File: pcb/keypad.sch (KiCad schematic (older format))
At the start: 1 part

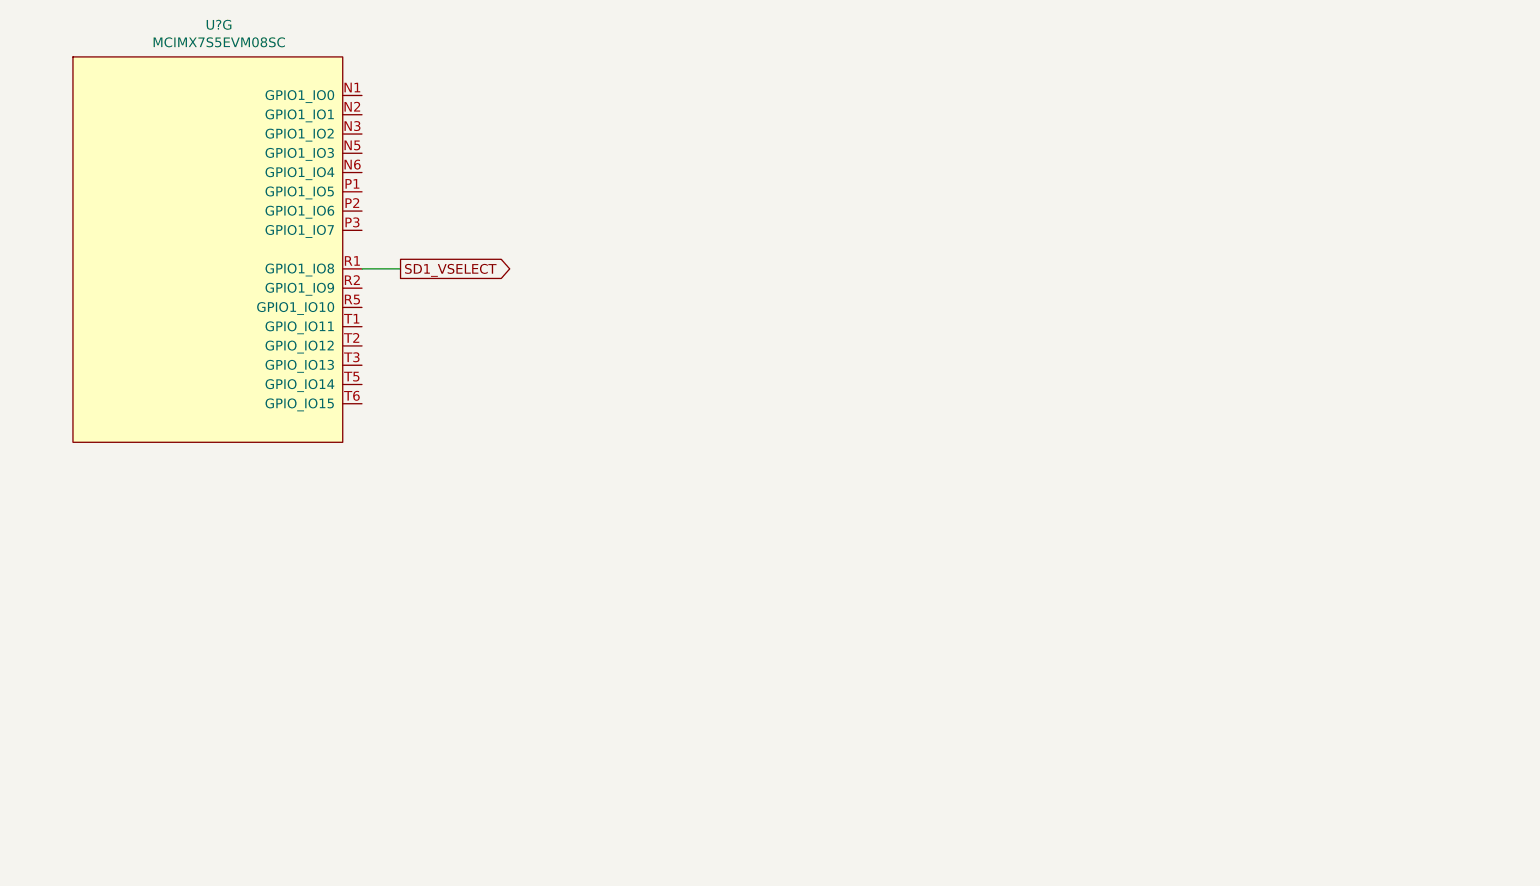
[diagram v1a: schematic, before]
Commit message: pcb: finishing sch for r0.1
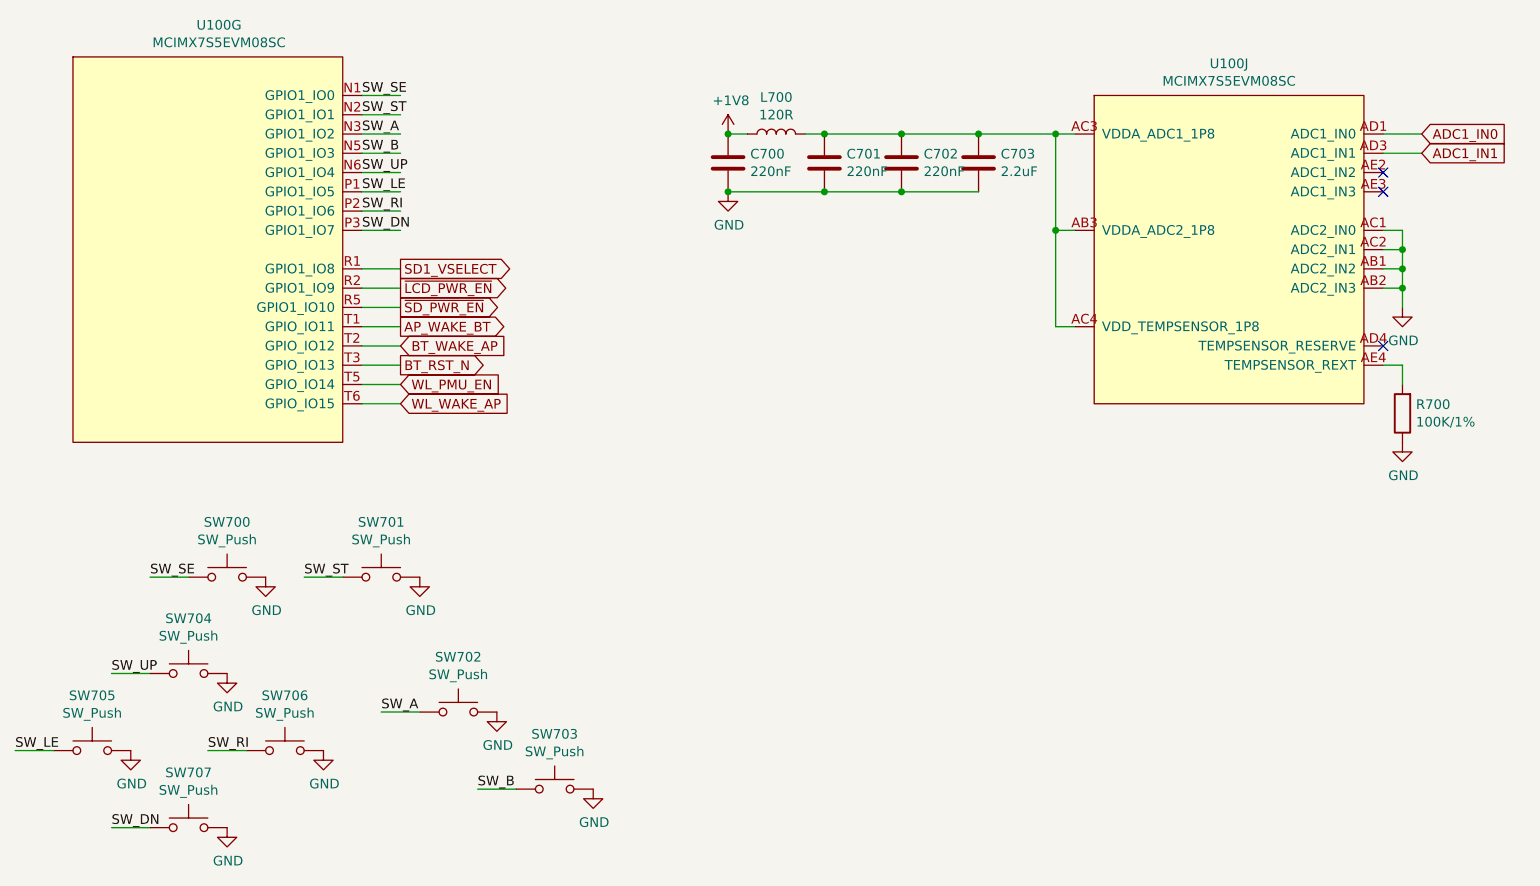
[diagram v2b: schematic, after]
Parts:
- added C700, C701, C702: 220nF, Capacitor_SMD:C_0402_1005Metric, symbol Device:C
- added C703: 2.2uF, Capacitor_SMD:C_0402_1005Metric, symbol Device:C
- added L700: 120R, Inductor_SMD:L_0603_1608Metric, symbol Device:L
- added R700: 100K/1%, Resistor_SMD:R_0603_1608Metric, symbol Device:R
- added SW700, SW701, SW702, SW703, SW704, SW705, SW706, SW707: SW_Push, footprints:contact, symbol Switch:SW_Push
- added unit 10 of U100
- U100: renamed from U?; footprint (none) -> footprints:BGA-541_25x25_19.0x19.0mm
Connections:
- net labels added: +1V8, ADC1_IN0, ADC1_IN1, AP_WAKE_BT, BT_RST_N, BT_WAKE_AP, GND, SW_A, SW_B, SW_DN, SW_LE, SW_RI, SW_SE, SW_ST, SW_UP, WL_PMU_EN, WL_WAKE_AP, ~LCD_PWR_EN, ~SD_PWR_EN
- wire segments 1 -> 49
- no-connect marks 0 -> 3
